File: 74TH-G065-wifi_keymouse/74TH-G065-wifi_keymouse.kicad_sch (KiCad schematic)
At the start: 21 parts, among them J1 USB_TypeA-2.0_Plug, J2 ESP-Prog-ProgramCOM_RECV, J3 ESP-Prog-ProgramCOM_RECV_Stra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, SW1 SW_Push, U1 CH9329, U2 ESP32-C3-WROOM-02, U3 CH217K, U4 AMS1117

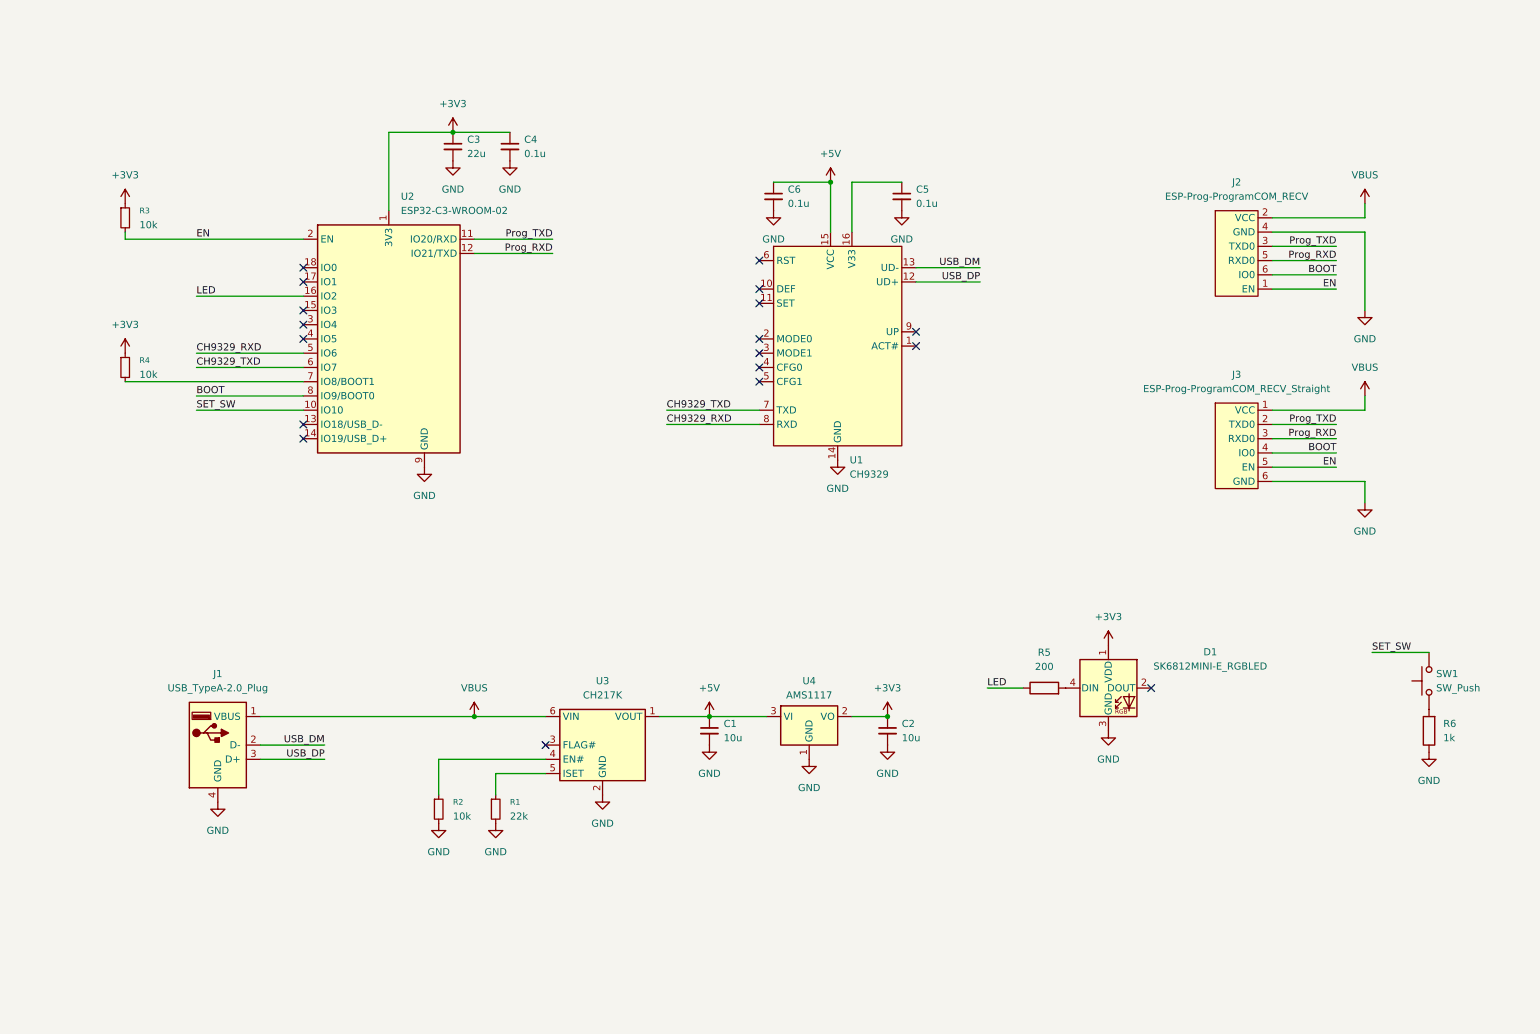
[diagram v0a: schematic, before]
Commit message: wifi_keymouse/1.0.0
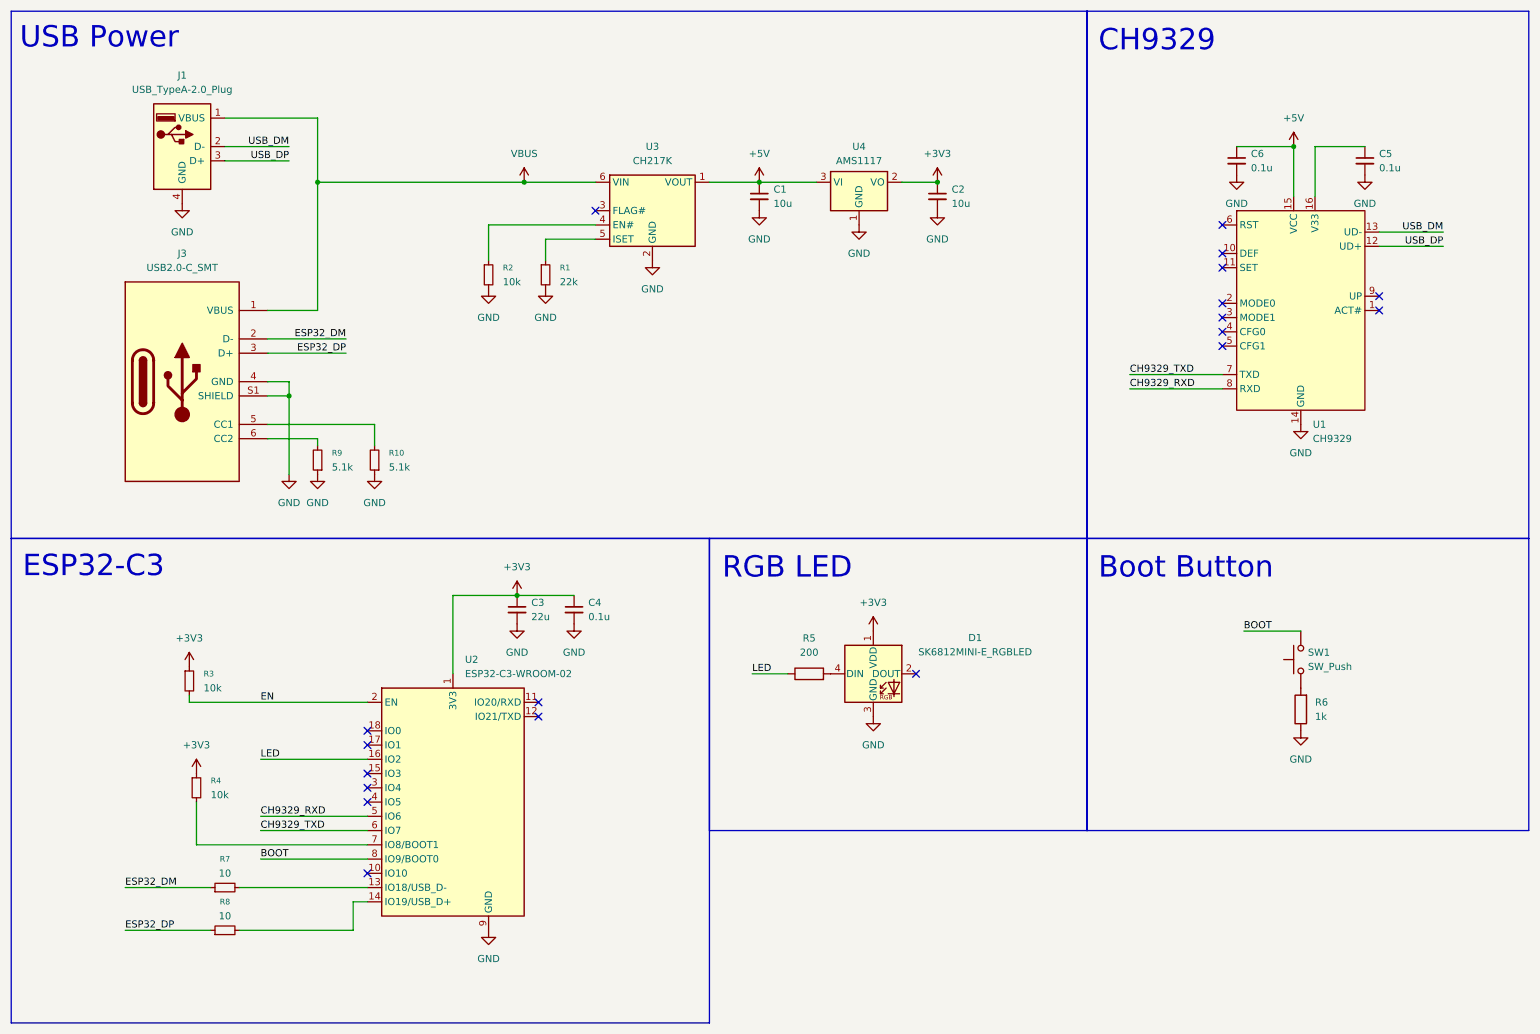
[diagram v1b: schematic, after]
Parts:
- removed J2: ESP-Prog-ProgramCOM_RECV, 74th:Connector_BoxPinHeader_2x03_P1.27mm, symbol 74th_Interface:ESP-Prog-ProgramCOM_RECV
- removed J3: ESP-Prog-ProgramCOM_RECV_Straight, 74th:PinOut_Pin_6_GND, symbol 74th_Interface:ESP-Prog-ProgramCOM_RECV_Straight
- added J3: USB2.0-C_SMT, 74th:Connector_USB-C-Receptacle_SMT_12-Pin_Simple, symbol 74th_Interface:USB_TypeC-2.0_Receptacle_Simple
- added R10, R9: 5.1k, 74th:Register_0603_1608, symbol Device:R_Small
- added R7, R8: 10, 74th:Register_0603_1608, symbol Device:R_Small
- SW1: Function (none) -> Boot
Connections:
- net BOOT: now also SW1.2
- net GND: now also J3.4 (GND), J3.S1 (SHIELD), R10.1, R9.1
- net VBUS: now also J3.1 (VBUS)
- net at U2.13 (IO18/USB_D-): now also R7.2
- net at U2.14 (IO19/USB_D+): now also R8.2
- net Prog_RXD: no longer names the net of U2.12 (IO21/TXD)
- net Prog_TXD: no longer names the net of U2.11 (IO20/RXD)
- net SET_SW: no longer names the net of U2.10 (IO10)
- net SET_SW: no longer SW1.2
- new net: J3.6 (CC2), R9.2
- new net: J3.5 (CC1), R10.2
- new net ESP32_DM: J3.2 (D-), R7.1
- new net ESP32_DP: J3.3 (D+), R8.1
- no-connect marks 18 -> 19
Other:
- note added: "Boot Button"
- note added: "CH9329"
- note added: "ESP32-C3"
- note added: "RGB LED"
- note added: "USB Power"
- moved on the sheet: C1, C2, C3, C4, C5, C6, D1, J1, R1, R2, R3, R4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
